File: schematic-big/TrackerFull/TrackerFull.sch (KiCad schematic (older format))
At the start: 60 parts, among them J1 Conn_01x05_Male, J2 MUC-20PFFR-JS7001, J3 Battery, J5 Conn_01x04_Male, J6 78727-0001, Q1 DMG2305UXQ, Q2 DMG2305UXQ, Q3 DMG2305UXQ, SW1 PTS647SK38SMTR2LFS, U1 TLV62585PDRLR, U2 LIS3DSH, U4 MCP73831-2-OT, U5 BGU8019, U6 U.FL, U7 MIC5232-2.8YD5, U8 ATtiny861A-MU

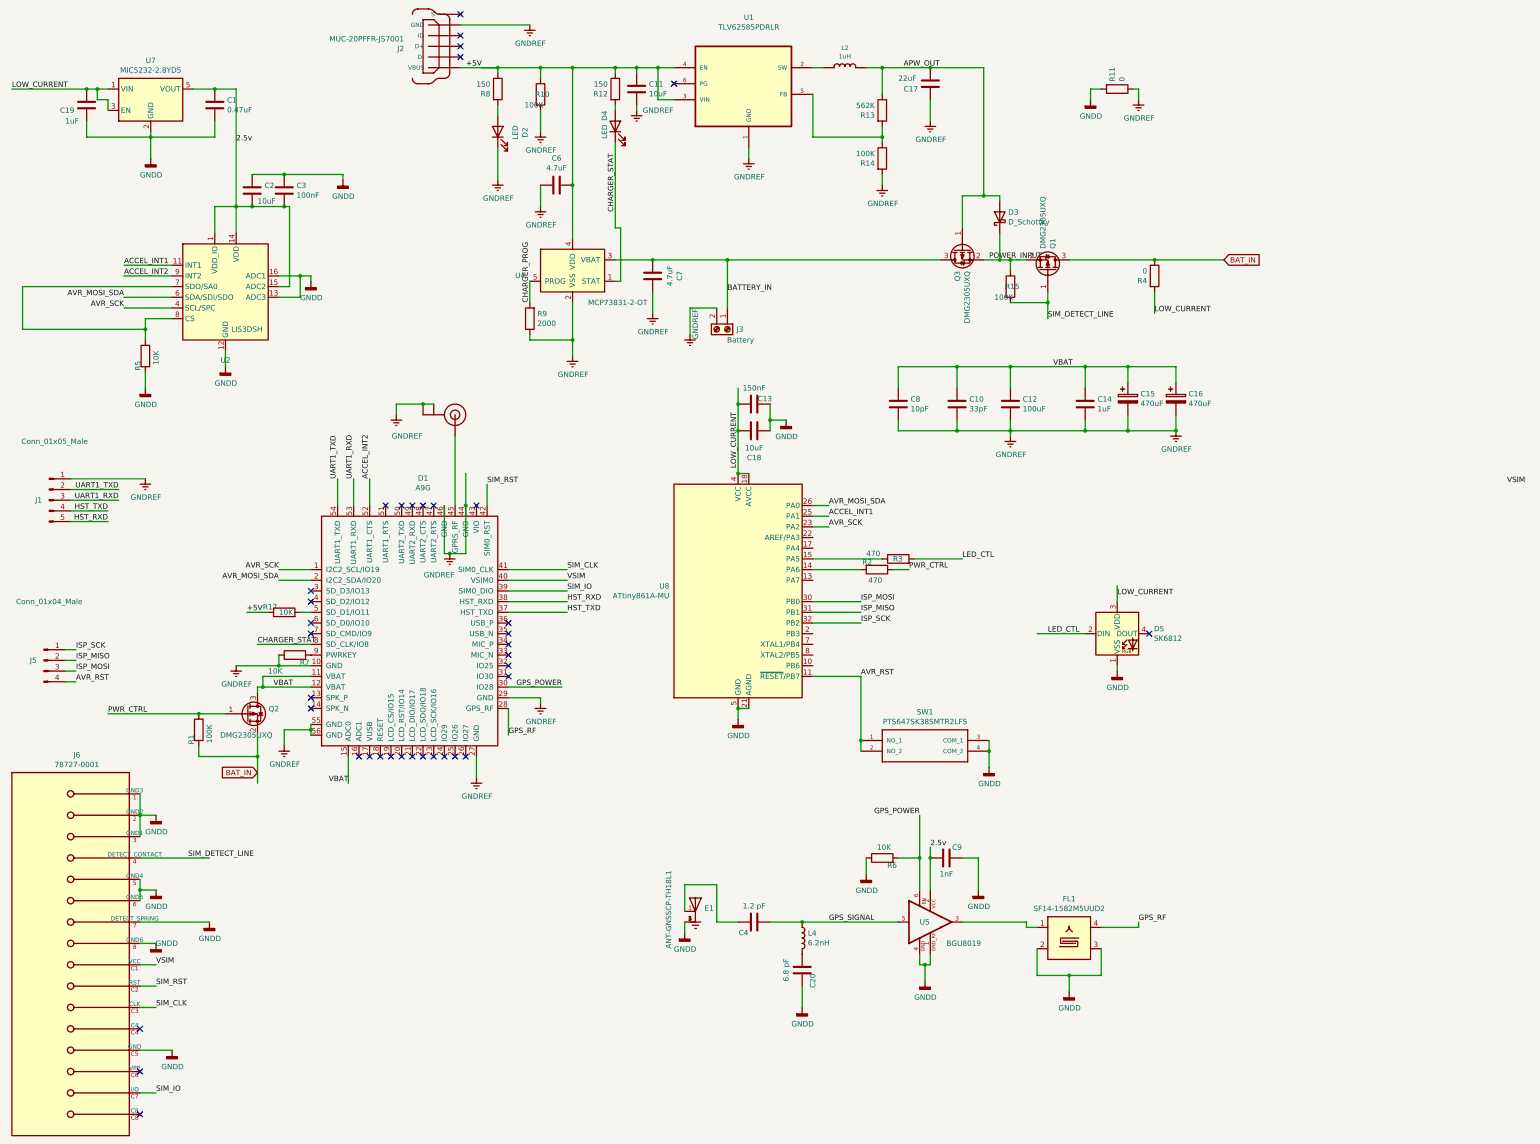
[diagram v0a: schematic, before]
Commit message: rf
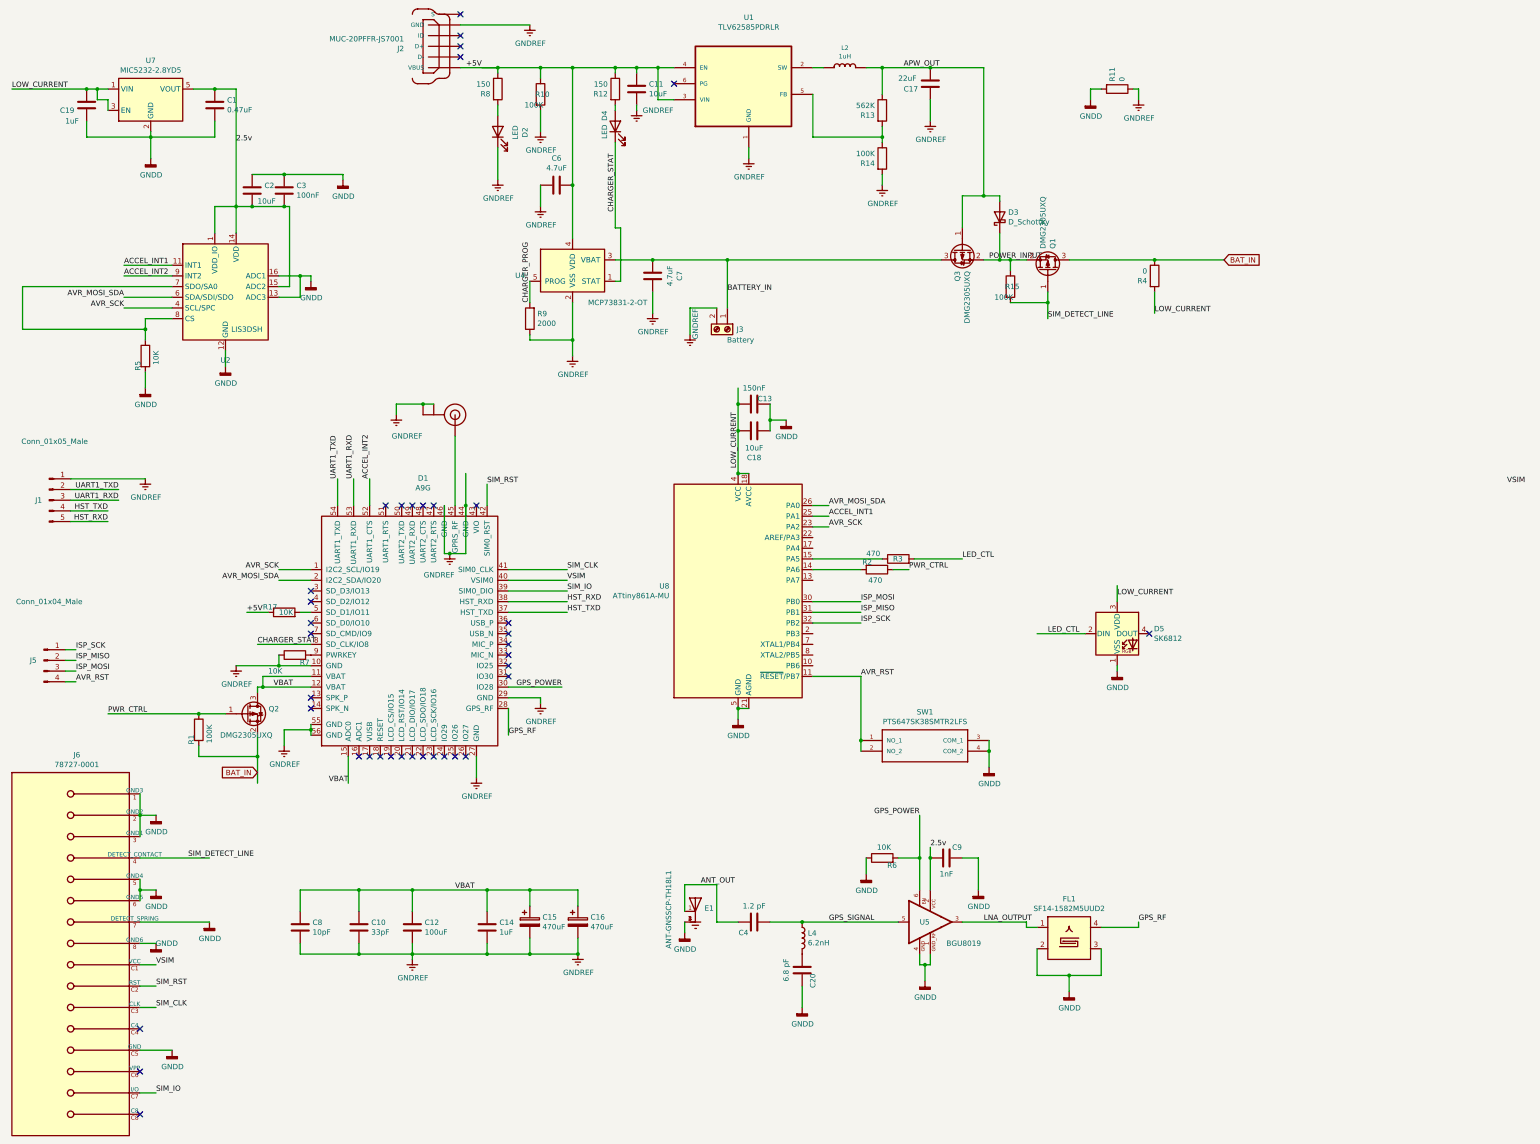
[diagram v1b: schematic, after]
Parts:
- C20: Поле5 (none) -> GRM1555C1E6R8CA01D
- C4: Поле5 (none) -> GRM1555C1H1R2BA01D
- C9: Поле5 (none) -> GRM1555C2A102JE01D
- L4: Поле5 (none) -> LQW15AN6N2B0ZD
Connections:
- net LNA_OUTPUT: now reaches FL1.1, U5.3
- net ANT_OUT: now reaches C4.2, E1.1
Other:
- moved on the sheet: C10, C12, C14, C15, C16, C8
